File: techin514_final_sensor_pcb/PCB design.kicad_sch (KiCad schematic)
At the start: 3 parts, among them SW1 SW_SPDT, U1 MOUDLE-SEEEDUINO-XIAO-ESP32C3, U2 BME280

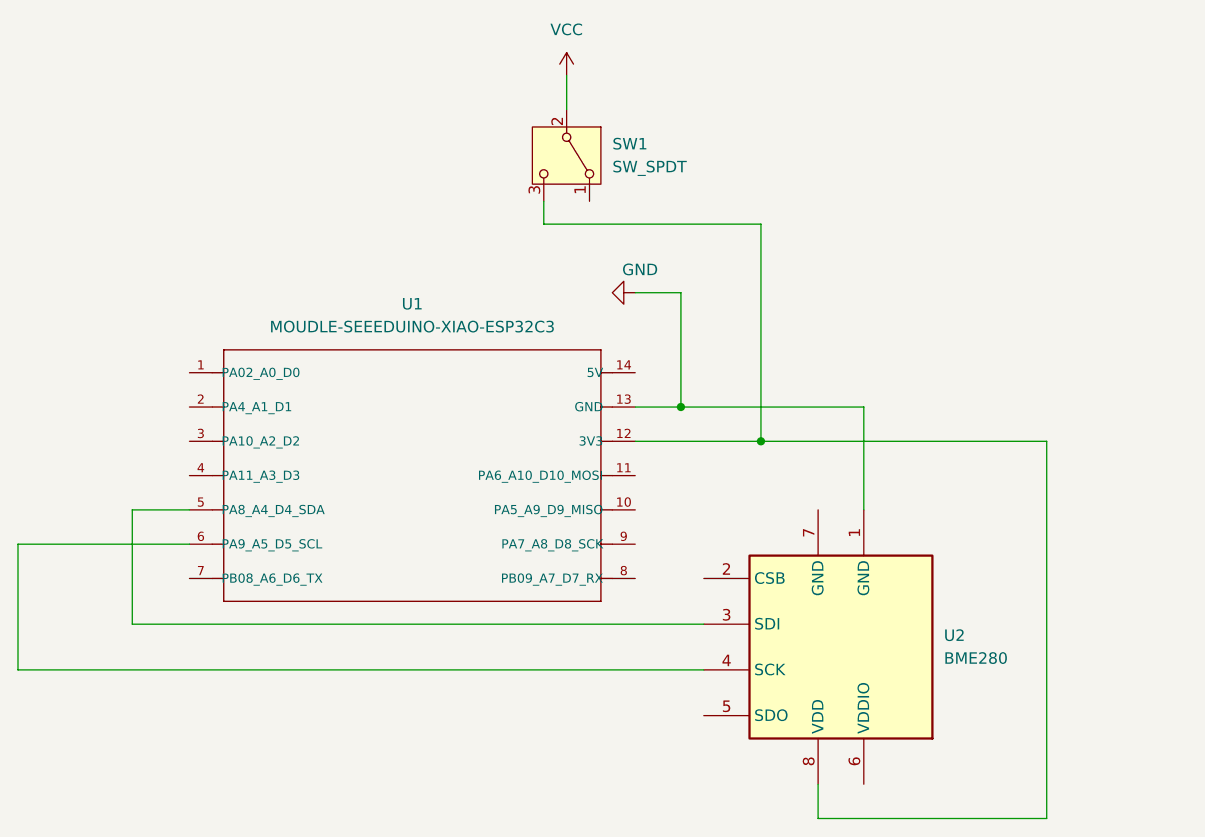
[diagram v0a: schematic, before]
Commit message: update
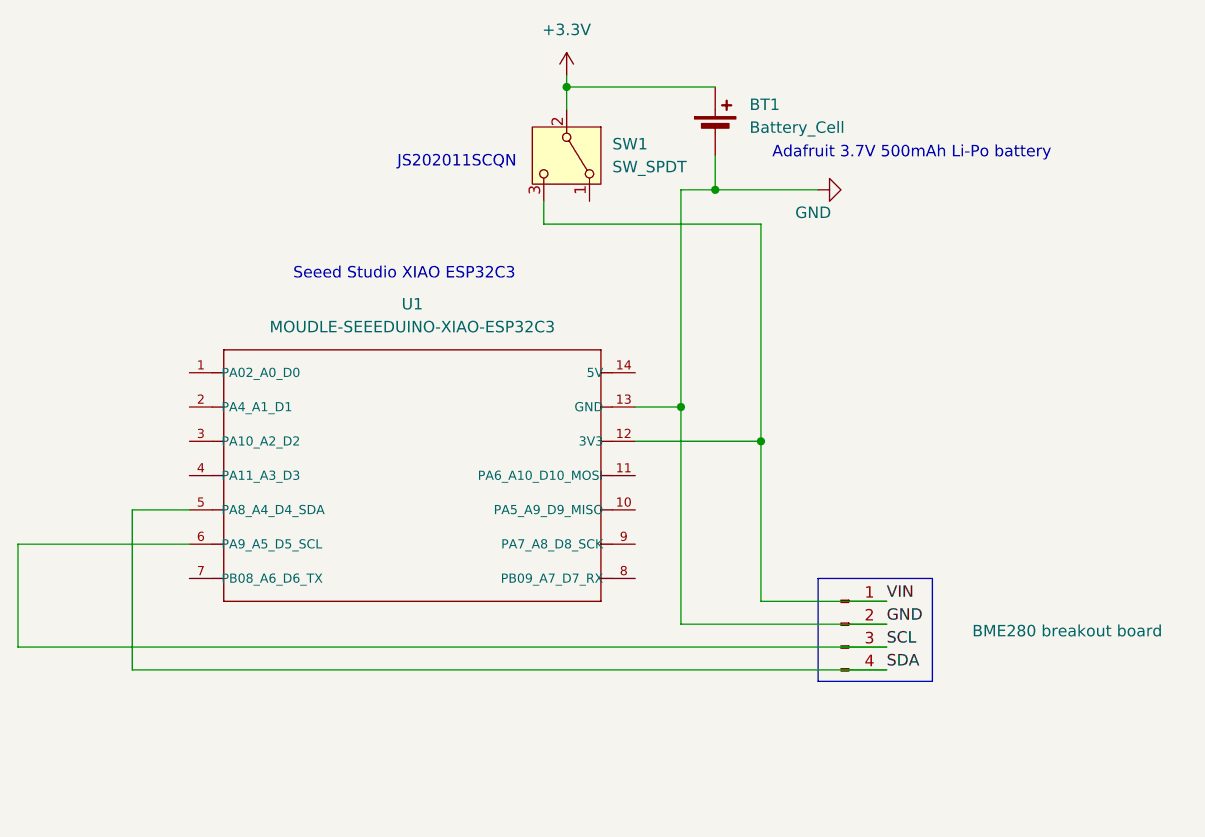
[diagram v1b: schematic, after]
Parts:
- removed U2: BME280, Package_LGA:Bosch_LGA-8_2.5x2.5mm_P0.65mm_ClockwisePinNumbering, symbol Sensor:BME280
- added BT1: Battery_Cell, Connector_JST:JST_PH_B2B-PH-K_1x02_P2.00mm_Vertical, symbol Device:Battery_Cell
- added J1: BME280 breakout board, Connector_PinHeader_2.54mm:PinHeader_1x04_P2.54mm_Vertical, symbol Connector:Conn_01x04_Pin
- SW1: footprint (none) -> Button_Switch_THT:SW_Slide-03_Wuerth-WS-SLTV_10x2.5x6.4_P2.54mm
- U1: footprint MOUDLE14P-SMD-2.54-21X17.8MM -> ESP32_xiao:MOUDLE14P-SMD-2.54-21X17.8MM
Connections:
- net GND: now also BT1.2 (-), J1.2 (Pin_2)
- net VIN: now reaches SW1.3 (C), U1.12 (3V3)
- net VIN: now also J1.1 (Pin_1)
- net SDA: now reaches U1.5 (PA8_A4_D4_SDA)
- net SDA: now also J1.4 (Pin_4)
- net SCL: now reaches U1.6 (PA9_A5_D5_SCL)
- net SCL: now also J1.3 (Pin_3)
- net VCC renamed +3.3V
- net +3.3V: now also BT1.1 (+)
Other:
- note added: "Adafruit 3.7V 500mAh Li-Po battery"
- note added: "JS202011SCQN"
- note added: "Seeed Studio XIAO ESP32C3"
